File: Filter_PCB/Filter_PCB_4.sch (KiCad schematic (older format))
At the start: 25 parts, among them J1 Conn_01x06_Male, J2 Conn_Coaxial, J3 Conn_Coaxial, U1 MCP4728

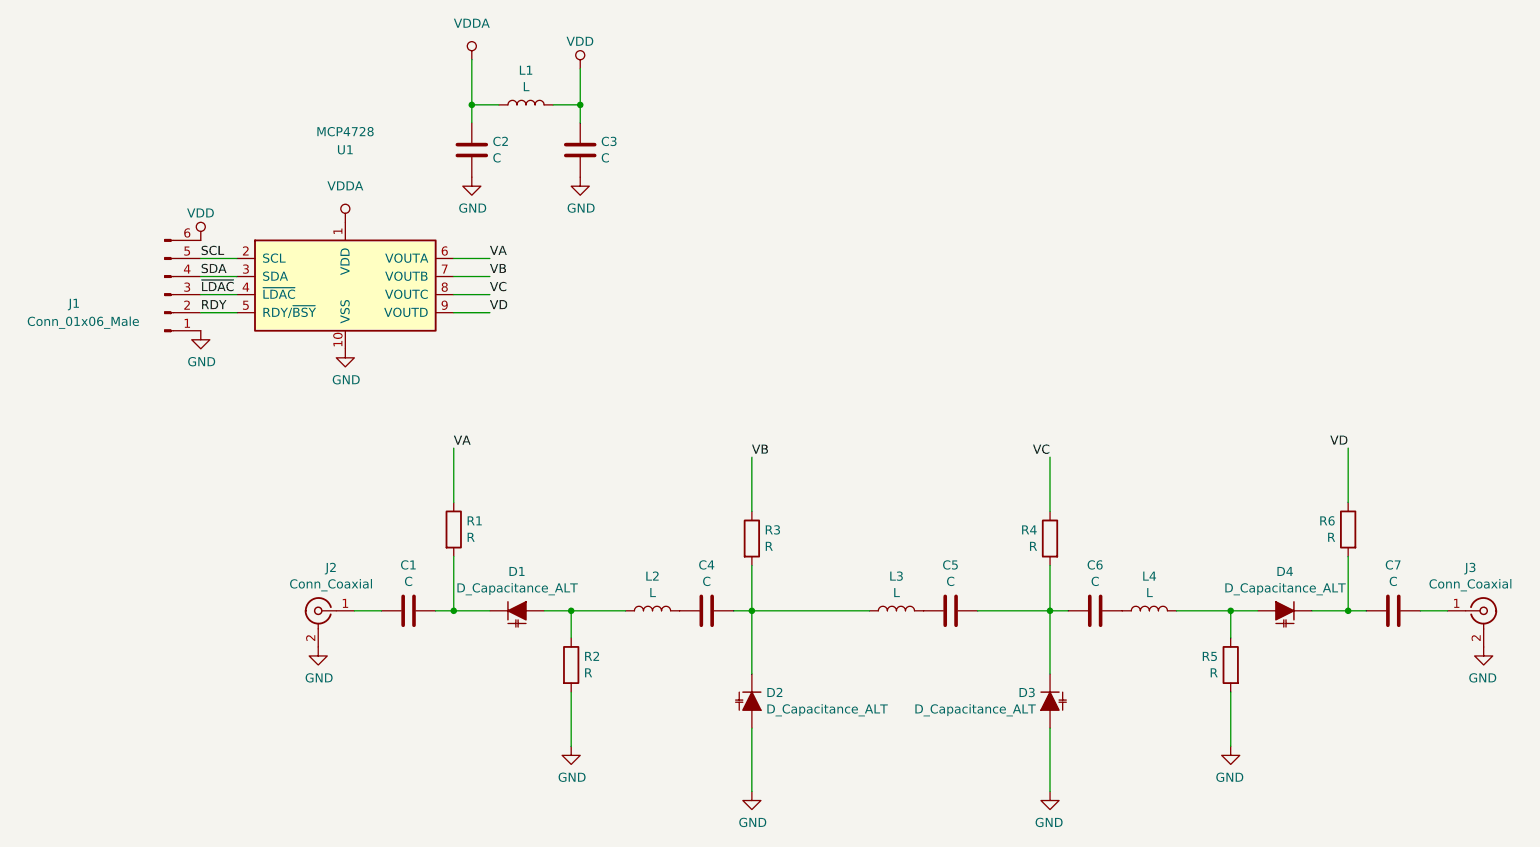
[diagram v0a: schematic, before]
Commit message: RF layout
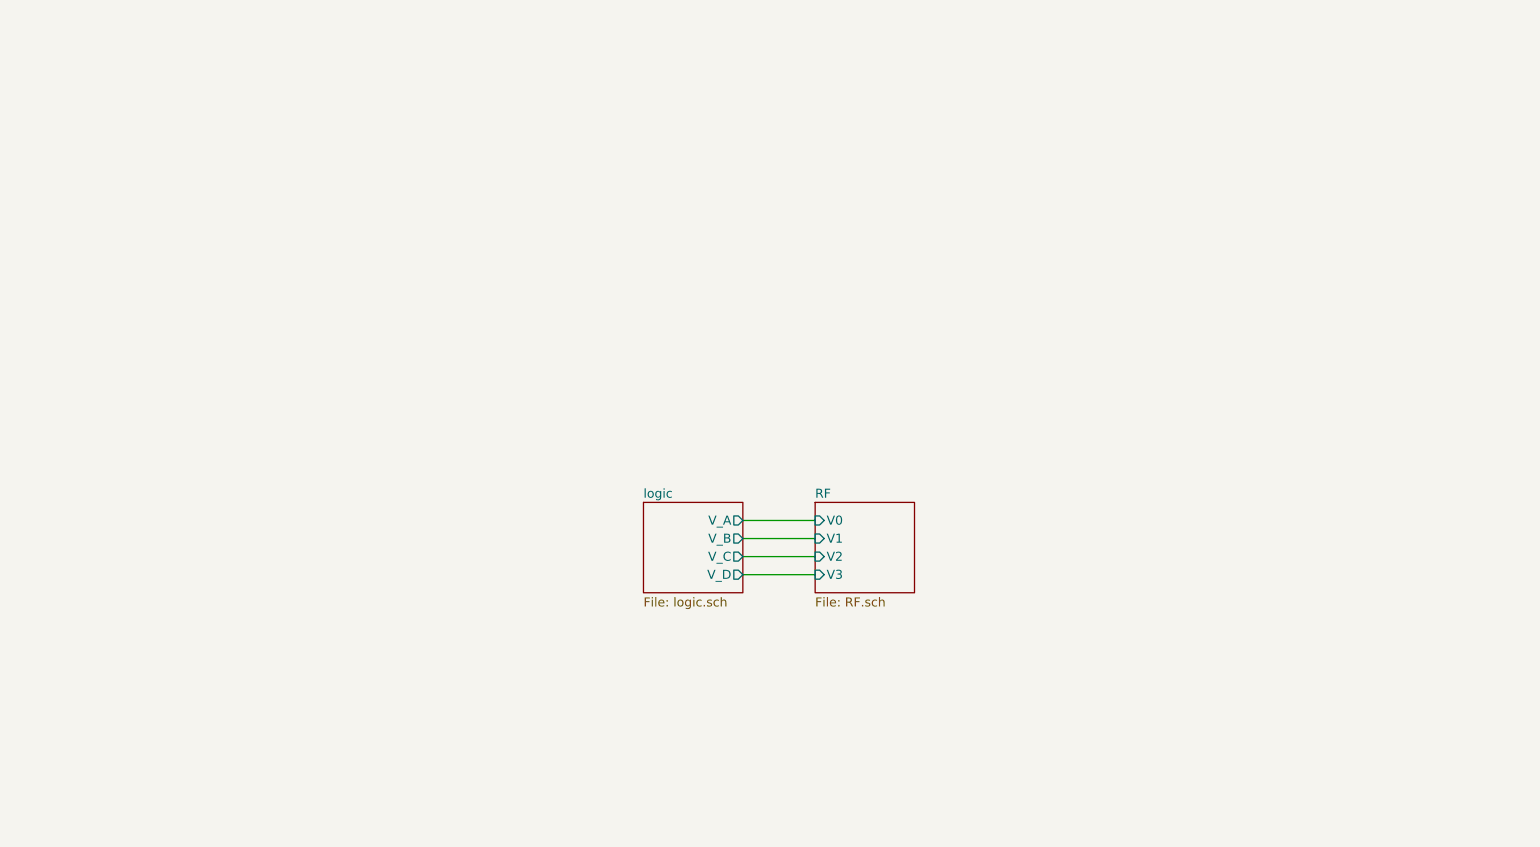
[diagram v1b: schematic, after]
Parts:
- removed C1, C2, C3, C4, C5, C6, C7: C, Capacitor_SMD:C_0603_1608Metric, symbol Device:C
- removed D1, D2, D3, D4: D_Capacitance_ALT, libs:D_SOD-523, symbol Device:D_Capacitance_ALT
- removed J1: Conn_01x06_Male, libs:SMD_1x06_P2.54mm_Horizontal, symbol Connector:Conn_01x06_Male
- removed J2, J3: Conn_Coaxial, libs:SMA_generic_EdgeMount, symbol Connector:Conn_Coaxial
- removed L1, L2, L3, L4: L, Inductor_SMD:L_0603_1608Metric, symbol Device:L
- removed R1, R2, R3, R4, R5, R6: R, Resistor_SMD:R_0603_1608Metric, symbol Device:R
- removed U1: MCP4728, Package_SO:MSOP-10_3x3mm_P0.5mm, symbol Analog_DAC:MCP4728
